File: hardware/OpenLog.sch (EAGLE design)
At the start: 19 parts, among them Q1 16MHZ, U1 ATMEGA328P_TQFP, U2 3.3V MIC5205, U3 microSD Socket

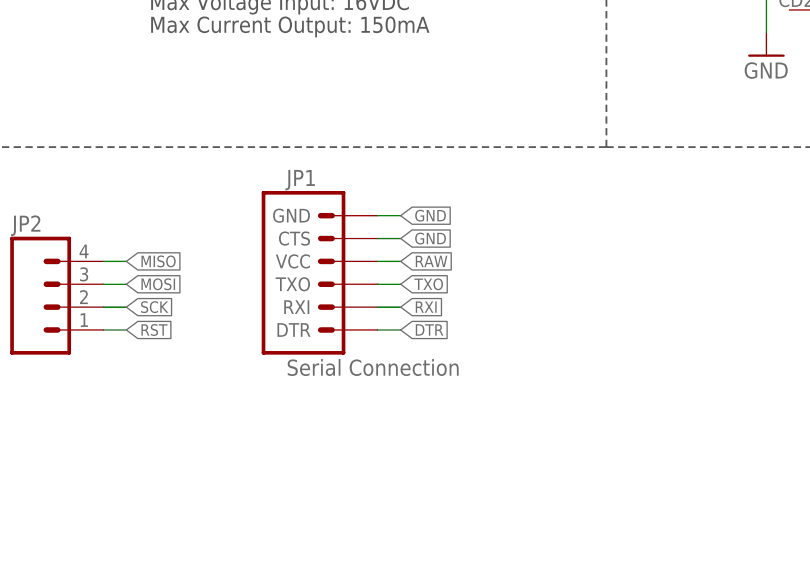
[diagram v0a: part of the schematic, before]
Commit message: Initial QC checklist run though
As in my own, before I actually get one done.
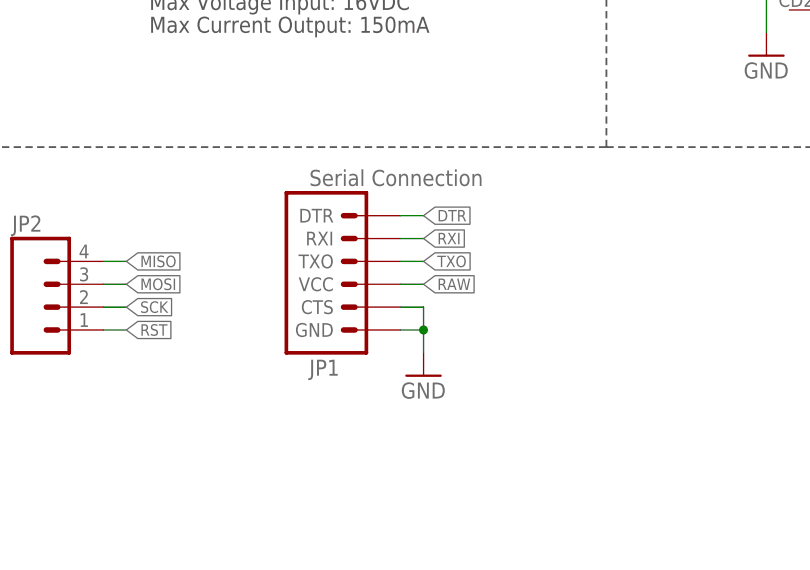
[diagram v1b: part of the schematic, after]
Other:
- moved on the sheet: JP1
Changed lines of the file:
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@@
 <part name="FID1" library="SparkFun-Aesthetics" deviceset="FIDUCIAL" device="UFIDUCIAL"/>
 <part name="FID2" library="SparkFun-Aesthetics" deviceset="FIDUCIAL" device="UFIDUCIAL"/>
+<part name="GND6" library="SparkFun" deviceset="GND" device=""/>
 </parts>
 <sheets>
@@
 <instance part="P+1" gate="G$1" x="167.64" y="165.1"/>
 <instance part="GND5" gate="1" x="167.64" y="101.6"/>
-<instance part="JP1" gate="G$1" x="43.18" y="93.98"/>
+<instance part="JP1" gate="G$1" x="45.72" y="96.52" rot="MR180"/>
 <instance part="C2" gate="G$1" x="147.32" y="162.56" smashed="yes" rot="R270">
 <attribute name="NAME" x="147.193" y="163.576" size="1.778" layer="95" rot="R90"/>
@@
 <instance part="FID1" gate="G$1" x="246.38" y="33.02"/>
 <instance part="FID2" gate="G$1" x="241.3" y="33.02"/>
+<instance part="GND6" gate="1" x="53.34" y="83.82"/>
 </instances>
 <busses>
@@
 </segment>
 <segment>
-<wire x1="48.26" y1="99.06" x2="50.8" y2="99.06" width="0.1524" layer="91"/>
+<wire x1="53.34" y1="88.9" x2="53.34" y2="86.36" width="0.1524" layer="91"/>
+<pinref part="GND6" gate="1" pin="GND"/>
+<wire x1="50.8" y1="91.44" x2="53.34" y2="91.44" width="0.1524" layer="91"/>
+<wire x1="53.34" y1="91.44" x2="53.34" y2="88.9" width="0.1524" layer="91"/>
 <pinref part="JP1" gate="G$1" pin="CTS"/>
-<label x="50.8" y="99.06" size="1.27" layer="95" xref="yes"/>
-</segment>
-<segment>
-<wire x1="48.26" y1="101.6" x2="50.8" y2="101.6" width="0.1524" layer="91"/>
 <pinref part="JP1" gate="G$1" pin="GND"/>
-<label x="50.8" y="101.6" size="1.27" layer="95" xref="yes"/>
+<wire x1="50.8" y1="88.9" x2="53.34" y2="88.9" width="0.1524" layer="91"/>
+<junction x="53.34" y="88.9"/>
 </segment>
 <segment>
@@
 </segment>
 <segment>
-<wire x1="48.26" y1="93.98" x2="50.8" y2="93.98" width="0.1524" layer="91"/>
+<wire x1="50.8" y1="96.52" x2="53.34" y2="96.52" width="0.1524" layer="91"/>
 <pinref part="JP1" gate="G$1" pin="TXO"/>
-<label x="50.8" y="93.98" size="1.27" layer="95" xref="yes"/>
+<label x="53.34" y="96.52" size="1.27" layer="95" rot="MR180" xref="yes"/>
 </segment>
 </net>
@@
 </segment>
 <segment>
-<wire x1="48.26" y1="96.52" x2="50.8" y2="96.52" width="0.1524" layer="91"/>
+<wire x1="50.8" y1="93.98" x2="53.34" y2="93.98" width="0.1524" layer="91"/>
 <pinref part="JP1" gate="G$1" pin="VCC"/>
-<label x="50.8" y="96.52" size="1.27" layer="95" xref="yes"/>
+<label x="53.34" y="93.98" size="1.27" layer="95" rot="MR180" xref="yes"/>
 </segment>
 </net>
@@
 <net name="DTR" class="0">
 <segment>
-<wire x1="48.26" y1="88.9" x2="50.8" y2="88.9" width="0.1524" layer="91"/>
+<wire x1="50.8" y1="101.6" x2="53.34" y2="101.6" width="0.1524" layer="91"/>
 <pinref part="JP1" gate="G$1" pin="DTR"/>
-<label x="50.8" y="88.9" size="1.27" layer="95" xref="yes"/>
+<label x="53.34" y="101.6" size="1.27" layer="95" rot="MR180" xref="yes"/>
 </segment>
 <segment>
@@
 </segment>
 <segment>
-<wire x1="48.26" y1="91.44" x2="50.8" y2="91.44" width="0.1524" layer="91"/>
+<wire x1="50.8" y1="99.06" x2="53.34" y2="99.06" width="0.1524" layer="91"/>
 <pinref part="JP1" gate="G$1" pin="RXI"/>
-<label x="50.8" y="91.44" size="1.27" layer="95" xref="yes"/>
-</segment>
-</net>
+<label x="53.34" y="99.06" size="1.27" layer="95" rot="MR180" xref="yes"/>
+</segment>
+</net>
